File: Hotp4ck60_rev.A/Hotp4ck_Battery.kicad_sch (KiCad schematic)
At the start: 15 parts, among them Q1 AO3401A, SW2 SW_DIP_x01, U3 TP4056, U4 MAX17048

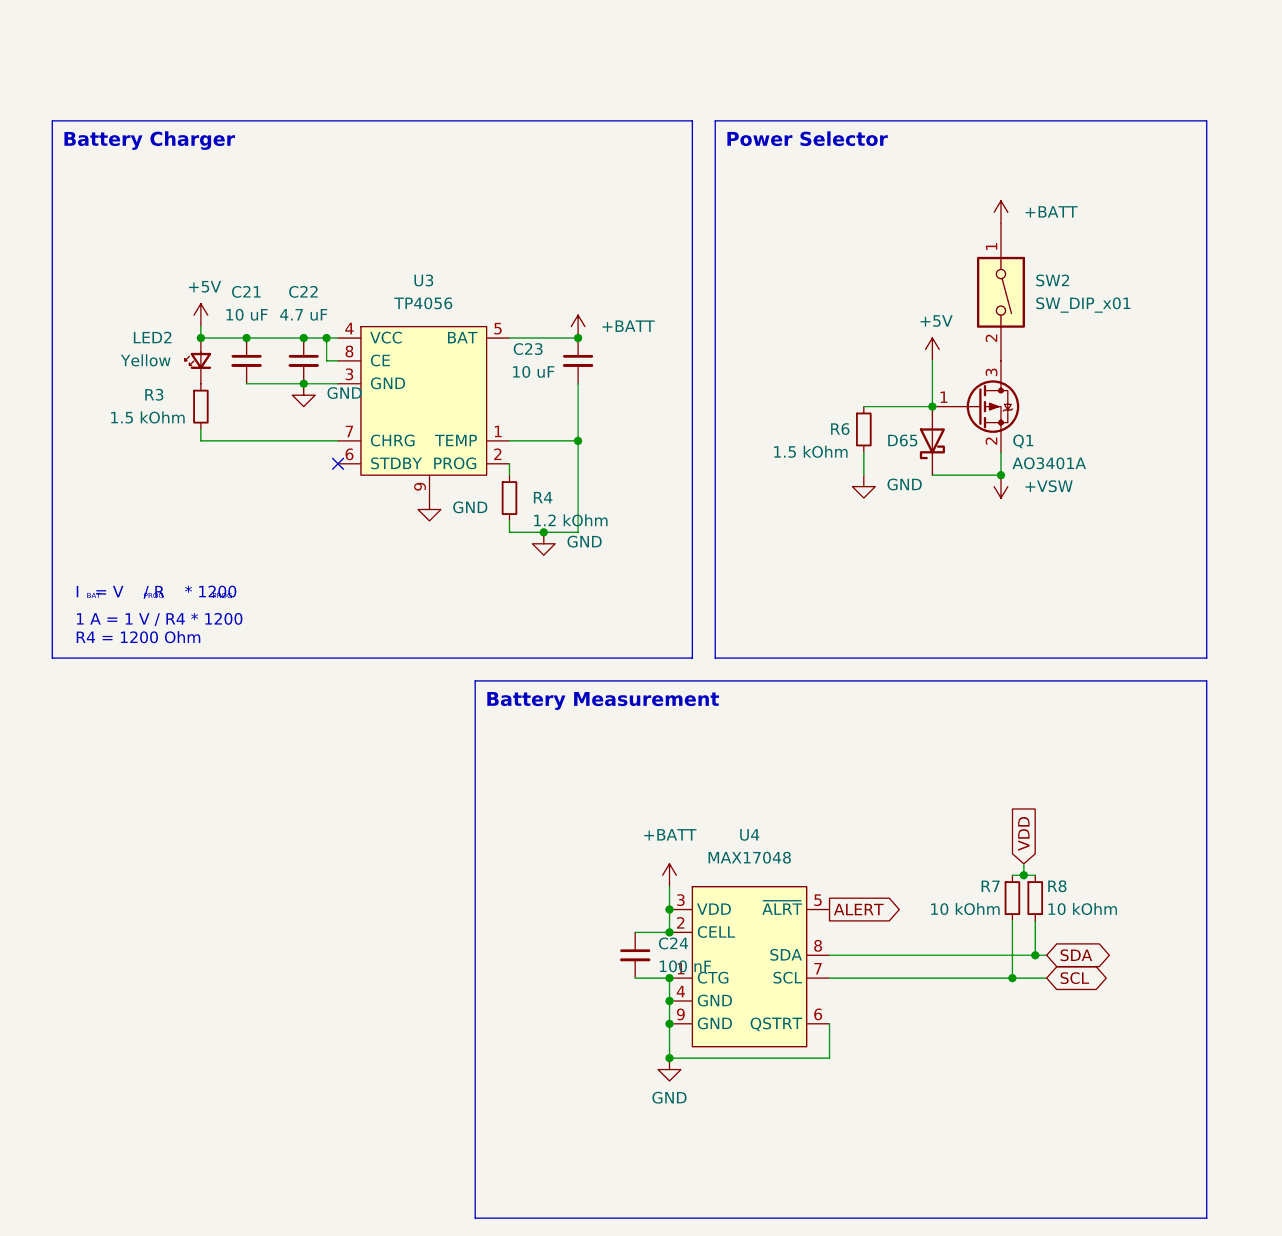
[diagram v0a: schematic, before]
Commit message: 배선 완료
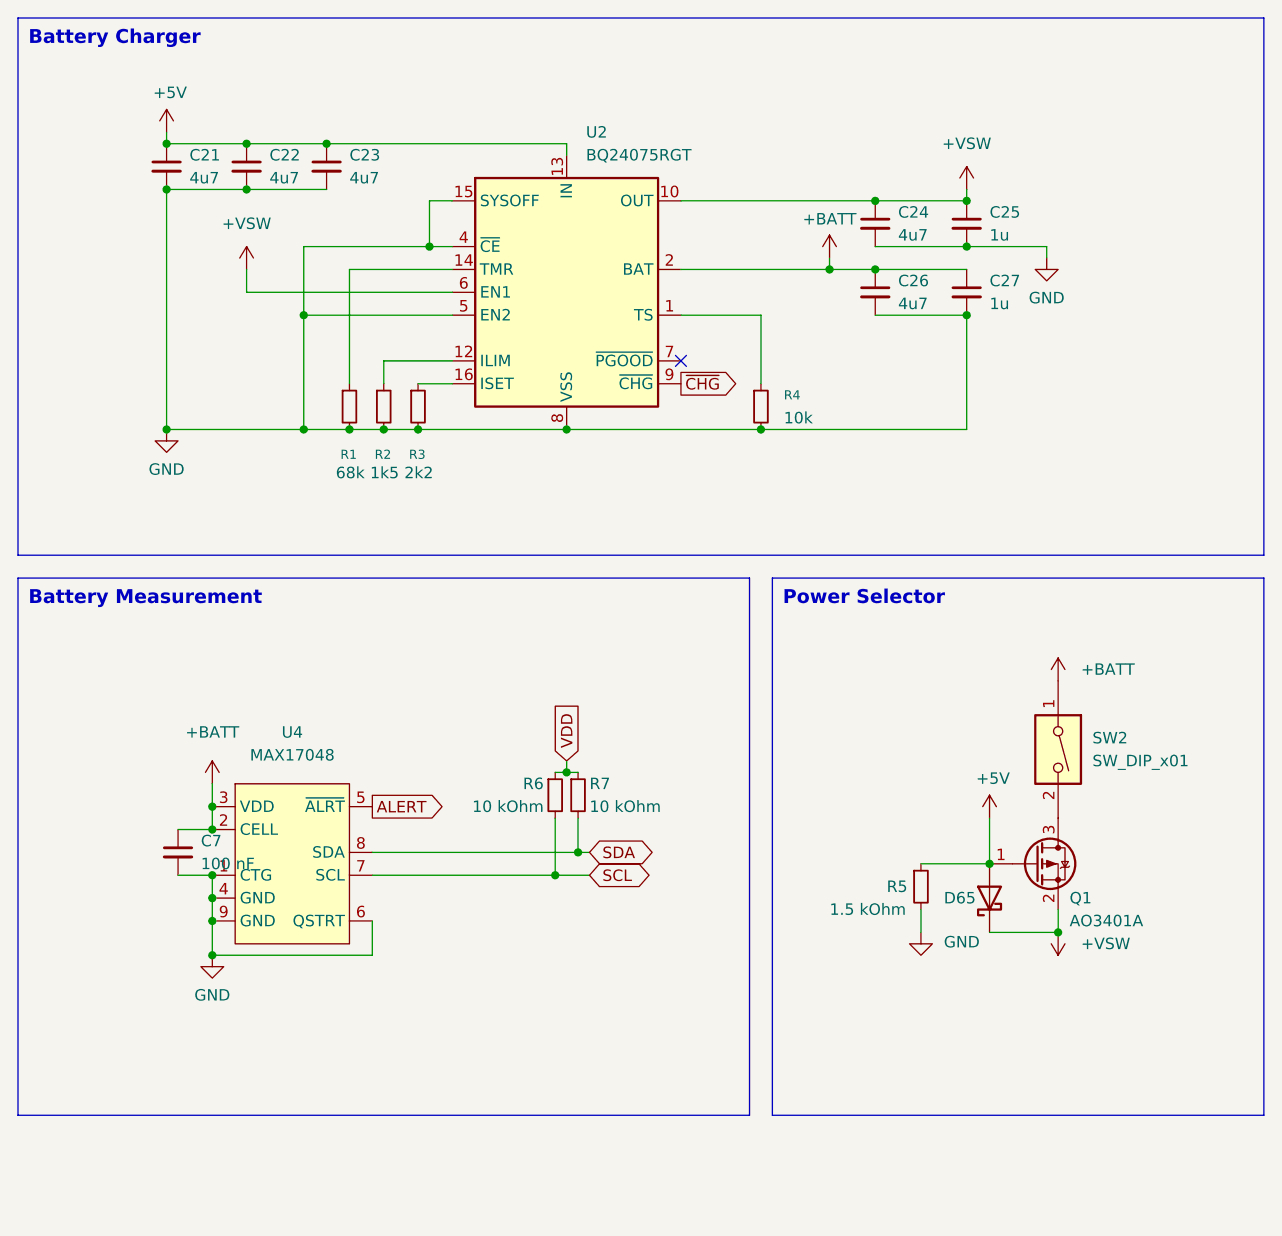
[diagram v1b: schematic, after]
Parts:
- removed LED2: Yellow, LED_SMD:LED_0603_1608Metric, symbol Device:LED_Small
- removed U3: TP4056, Package_SO:SOIC-8-1EP_3.9x4.9mm_P1.27mm_EP2.29x3mm, symbol marbastlib-various:TP4056
- added C24, C26: 4u7, Capacitor_SMD:C_0402_1005Metric, symbol Device:C_Small
- added C25, C27: 1u, Capacitor_SMD:C_0402_1005Metric, symbol Device:C_Small
- added R1: 68k, Resistor_SMD:R_0805_2012Metric, symbol Device:R_Small
- added R2: 1k5, Resistor_SMD:R_0402_1005Metric, symbol Device:R_Small
- added U2: BQ24075RGT, Package_DFN_QFN:VQFN-16-1EP_3x3mm_P0.5mm_EP1.6x1.6mm, symbol Battery_Management:BQ24075RGT
- C21, C23: value 10 uF -> 4u7; footprint Capacitor_SMD:C_0805_2012Metric -> Capacitor_SMD:C_0402_1005Metric; LCSC (none) -> C23733
- C22: value 4.7 uF -> 4u7; LCSC C52923 -> C23733; Notes X7R, 10% -> (none)
- R3: value 1.5 kOhm -> 2k2; LCSC C25792 -> C25879
- R4: value 1.2 kOhm -> 10k; LCSC C25867 -> C25744
- U4: now left out of the parts list
- renumbered C24 to C7, R6 to R5, R7 to R6, R8 to R7
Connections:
- net +5V: now also C23.1, U2.13 (IN)
- net +BATT: now also C26.1, C27.1, U2.2 (BAT), U2.3 (BAT); no longer C23.1
- net +VSW: now also C24.1, C25.1, U2.10 (OUT), U2.11 (OUT), U2.6 (EN1)
- net GND: now also R3.2, C24.2, C25.2, C26.2, C27.2, R1.2, R2.2, U2.15 (SYSOFF), U2.17 (VSS), U2.4 (~{CE}), U2.5 (EN2), U2.8 (VSS)
- net at R4.1: now also U2.1 (TS)
- net at R3.1: now also U2.16 (ISET)
- new net: R2.1, U2.12 (ILIM)
- new net: R1.1, U2.14 (TMR)
- new net ~{CHG}: U2.9 (~{CHG})
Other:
- note removed: "1 A = 1 V / R4 * 1200 R4 = 1200 Ohm"
- note removed: "BAT"
- note removed: "I = V / R * 1200"
- note removed: "PROG"
- moved on the sheet: C7, D65, Q1, R5, R6, R7, SW2, U4
